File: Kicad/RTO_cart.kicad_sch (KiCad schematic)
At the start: 17 parts, among them J1 2x22 card edge connector, J2 Oled 0.91" female, SW1 SW_Push, SW2 SW_Push, U1 74LS245, U2 74LS245, U3 74LS245, U4 Teensy4.1

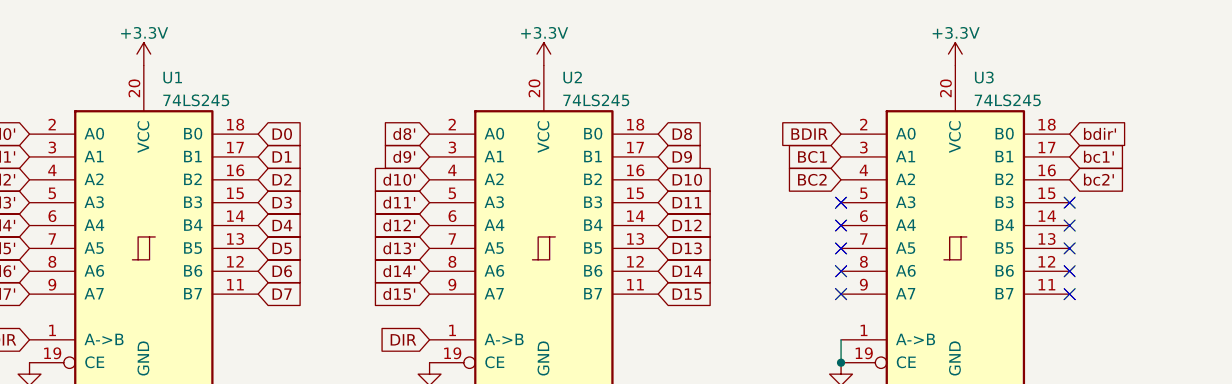
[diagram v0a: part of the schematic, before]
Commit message: Add files via upload
corrected the level shifter ICs to 74LVC245 instead of wrong typed 74LS245: WARNING! use only 74LVC245 chips, the other types could damage your Teensy becouse they output 5V instead of 3V3!
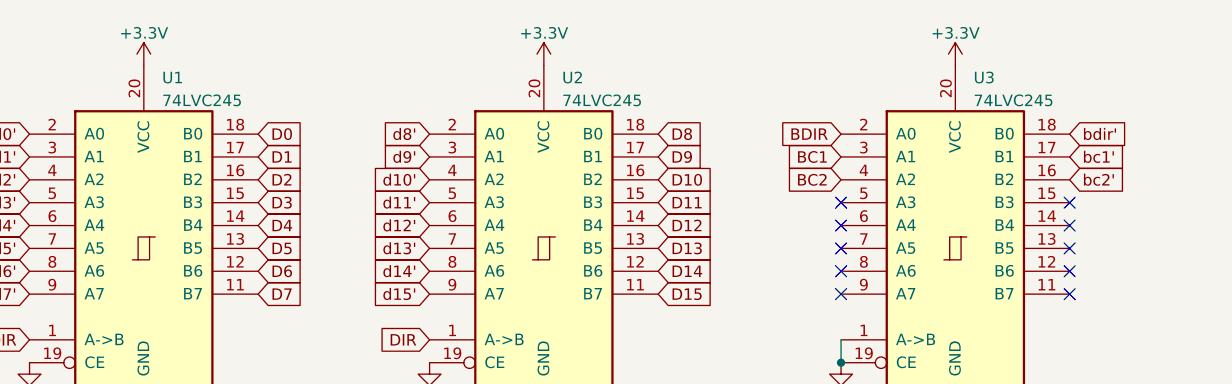
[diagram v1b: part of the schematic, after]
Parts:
- U1, U2, U3: value 74LS245 -> 74LVC245
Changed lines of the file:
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@@
       (effects (font (size 1.27 1.27)) (justify left))
     )
-    (property "Value" "74LS245" (id 1) (at 187.4394 31.8571 0)
+    (property "Value" "74LVC245" (id 1) (at 187.4394 31.8571 0)
       (effects (font (size 1.27 1.27)) (justify left))
     )
@@
       (effects (font (size 1.27 1.27)) hide)
     )
-    (property "Datasheet" "http://www.ti.com/lit/gpn/sn74LS245" (id 3) (at 185.42 48.26 0)
+    (property "Datasheet" "" (id 3) (at 185.42 48.26 0)
       (effects (font (size 1.27 1.27)) hide)
     )
@@
       (effects (font (size 1.27 1.27)) (justify left))
     )
-    (property "Value" "74LS245" (id 1) (at 97.2694 31.8571 0)
+    (property "Value" "74LVC245" (id 1) (at 97.2694 31.8571 0)
       (effects (font (size 1.27 1.27)) (justify left))
     )
@@
       (effects (font (size 1.27 1.27)) hide)
     )
-    (property "Datasheet" "http://www.ti.com/lit/gpn/sn74LS245" (id 3) (at 95.25 48.26 0)
+    (property "Datasheet" "" (id 3) (at 95.25 48.26 0)
       (effects (font (size 1.27 1.27)) hide)
     )
@@
       (effects (font (size 1.27 1.27)) (justify left))
     )
-    (property "Value" "74LS245" (id 1) (at 141.7194 31.8571 0)
+    (property "Value" "74LVC245" (id 1) (at 141.7194 31.8571 0)
       (effects (font (size 1.27 1.27)) (justify left))
     )
@@
       (effects (font (size 1.27 1.27)) hide)
     )
-    (property "Datasheet" "http://www.ti.com/lit/gpn/sn74LS245" (id 3) (at 139.7 48.26 0)
+    (property "Datasheet" "" (id 3) (at 139.7 48.26 0)
       (effects (font (size 1.27 1.27)) hide)
     )
@@
     )
     (path "/697b2099-5d1e-421b-86fb-66456fe646ee"
-      (reference "U1") (unit 1) (value "74LS245") (footprint "Package_DIP:DIP-20_W7.62mm_Socket")
+      (reference "U1") (unit 1) (value "74LVC245") (footprint "Package_DIP:DIP-20_W7.62mm_Socket")
     )
     (path "/6be8ebdc-952c-4ab9-8e80-82974edcb5f0"
-      (reference "U2") (unit 1) (value "74LS245") (footprint "Package_DIP:DIP-20_W7.62mm_Socket")
+      (reference "U2") (unit 1) (value "74LVC245") (footprint "Package_DIP:DIP-20_W7.62mm_Socket")
     )
     (path "/678e113b-998d-4fc9-b7c0-b0cd26248191"
-      (reference "U3") (unit 1) (value "74LS245") (footprint "Package_DIP:DIP-20_W7.62mm_Socket")
+      (reference "U3") (unit 1) (value "74LVC245") (footprint "Package_DIP:DIP-20_W7.62mm_Socket")
     )
     (path "/b76b3bdd-28ec-4a43-a3e2-5a3321ec7e57"
